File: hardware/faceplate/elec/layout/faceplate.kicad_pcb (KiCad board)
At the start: 2 copper layers, 181.9 x 127.5 mm, 65 parts

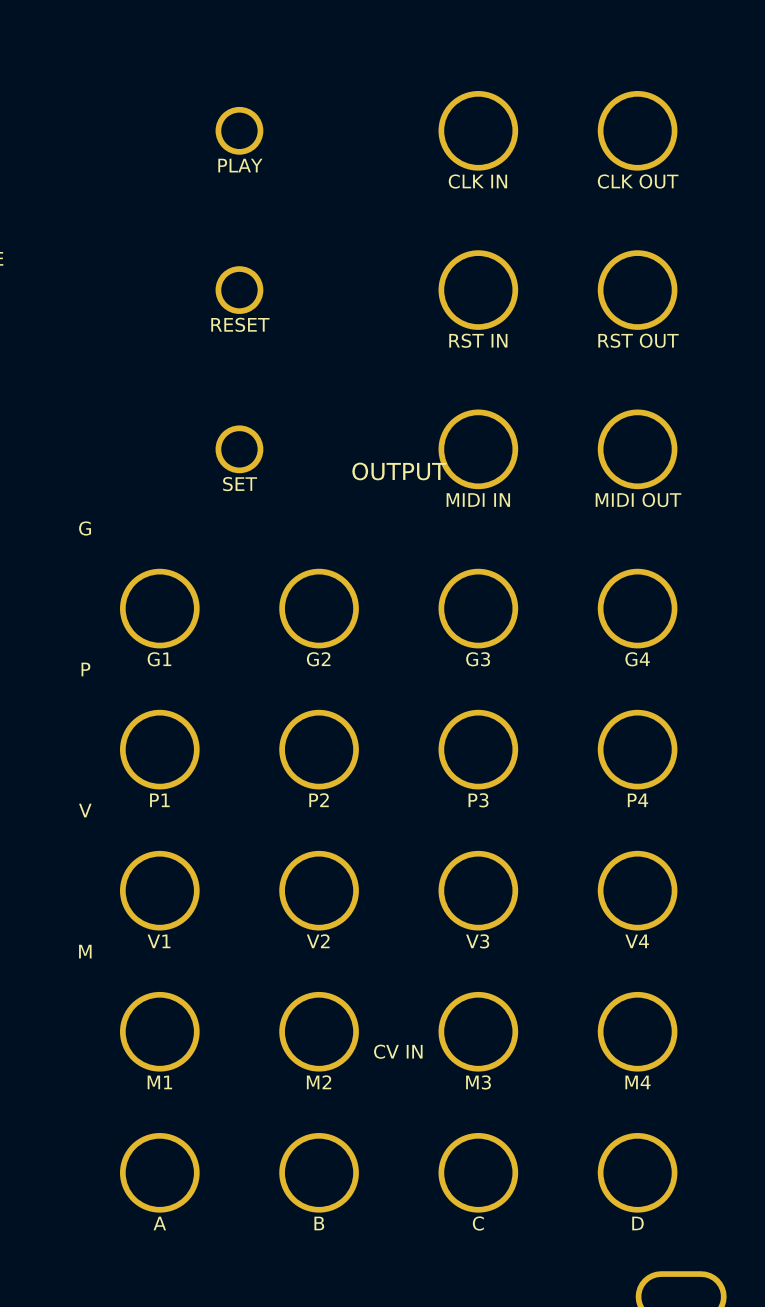
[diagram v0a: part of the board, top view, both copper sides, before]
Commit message: Routed
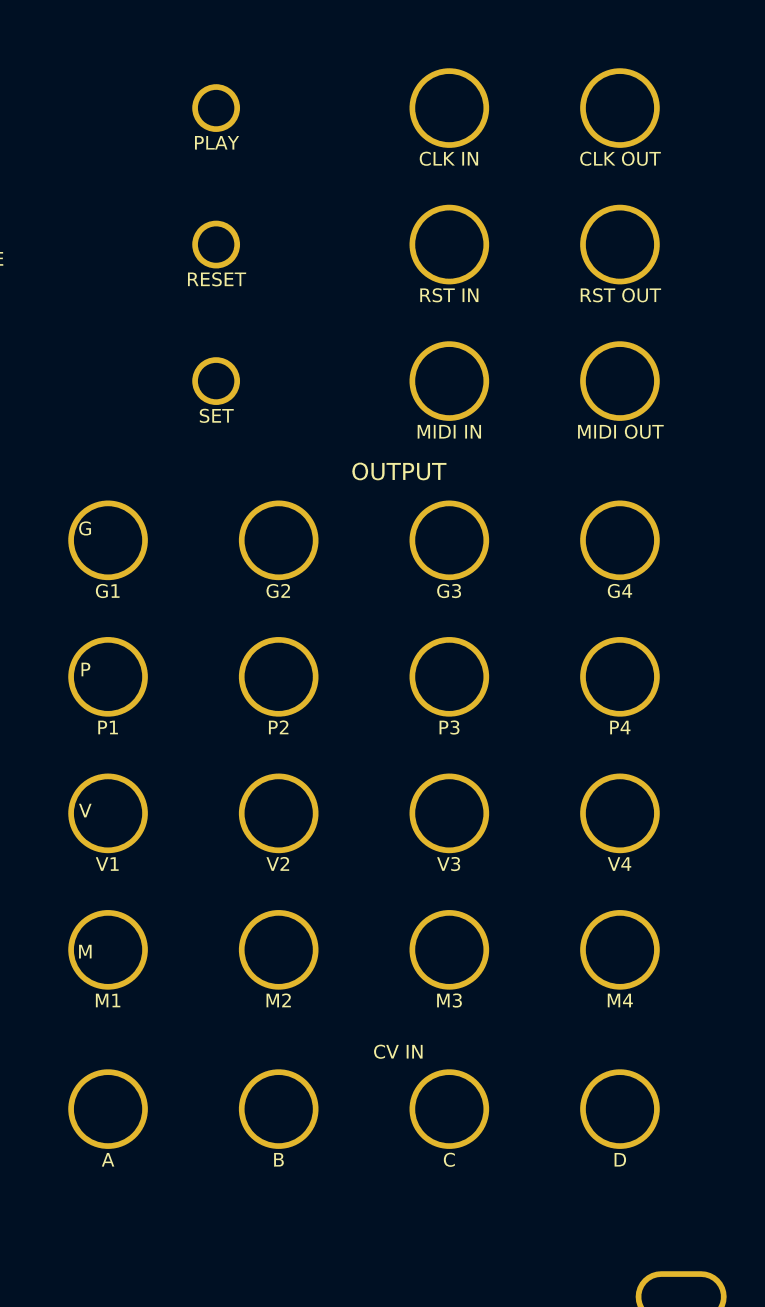
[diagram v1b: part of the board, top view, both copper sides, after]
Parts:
- moved J23 8.52 mm to (124.0, 94.0)
- moved J19 8.18 mm to (124.0, 82.0)
- moved J24 8.03 mm to (139.0, 94.0)
- moved J15 7.85 mm to (124.0, 70.0)
- moved J20 7.67 mm to (139.0, 82.0)
- moved J25 7.64 mm to (154.0, 94.0)
- moved J11 7.53 mm to (124.0, 58.0)
- moved J26 7.36 mm to (169.0, 94.0)
- moved J16 7.32 mm to (139.0, 70.0)
- moved J21 7.26 mm to (154.0, 82.0)
- moved J27 7.22 mm to (124.0, 108.0)
- moved J22 6.97 mm to (169.0, 82.0)
- moved J12 6.97 mm to (139.0, 58.0)
- moved J17 6.89 mm to (154.0, 70.0)
- moved J28 6.63 mm to (139.0, 108.0)
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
